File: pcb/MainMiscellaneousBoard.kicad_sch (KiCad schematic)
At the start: 7 parts, among them J4 S04B-PASK-2, J5 Conn_01x08, J6 Conn_01x08, J7 S04B-PASK-2, U1 ItsyBitsy_ESP32, U2 Seeed_Studio_XIAO-ESP32-S3-Se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

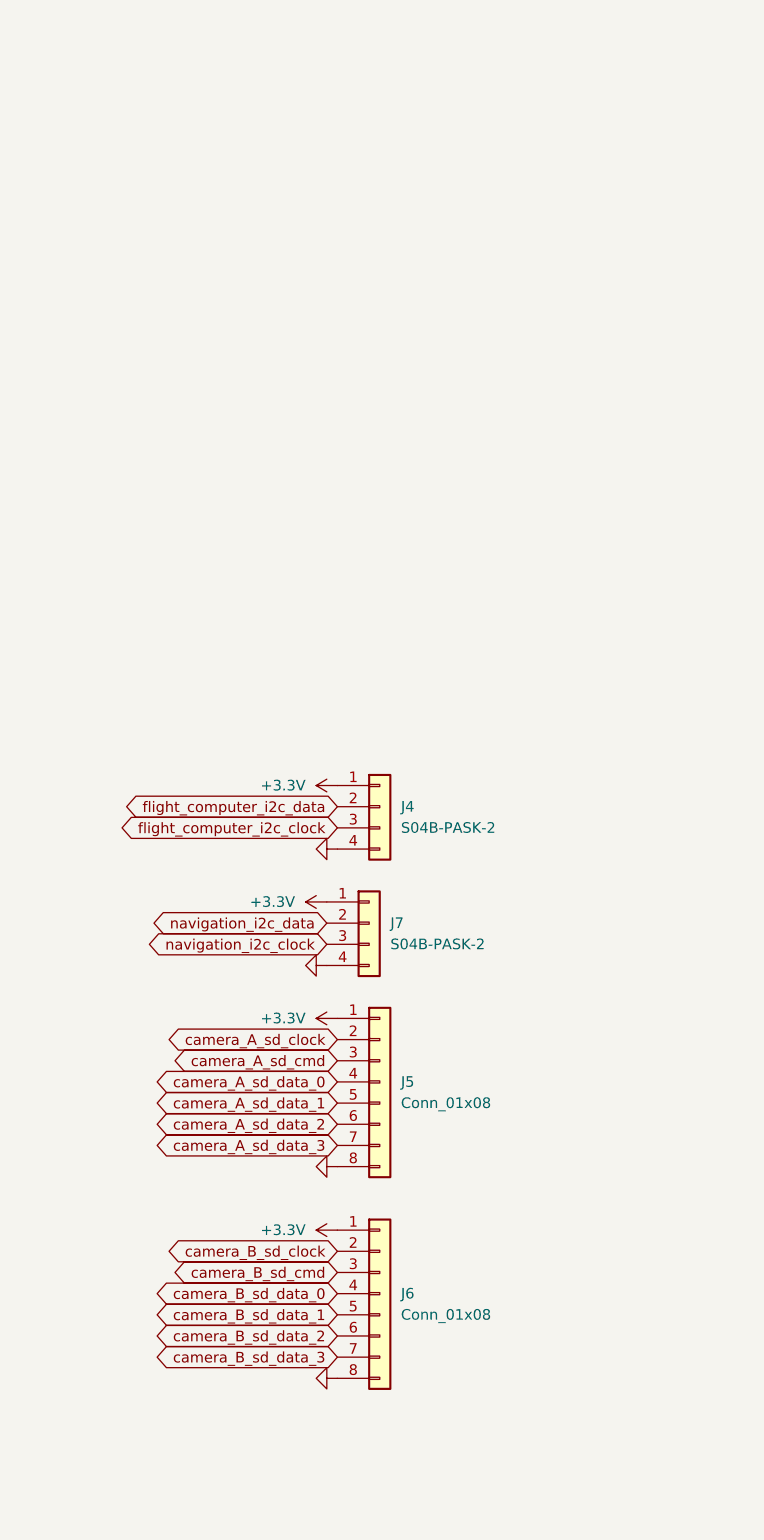
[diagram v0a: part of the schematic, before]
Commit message: Added edge connector for `MainMiscellaneousBoard`.
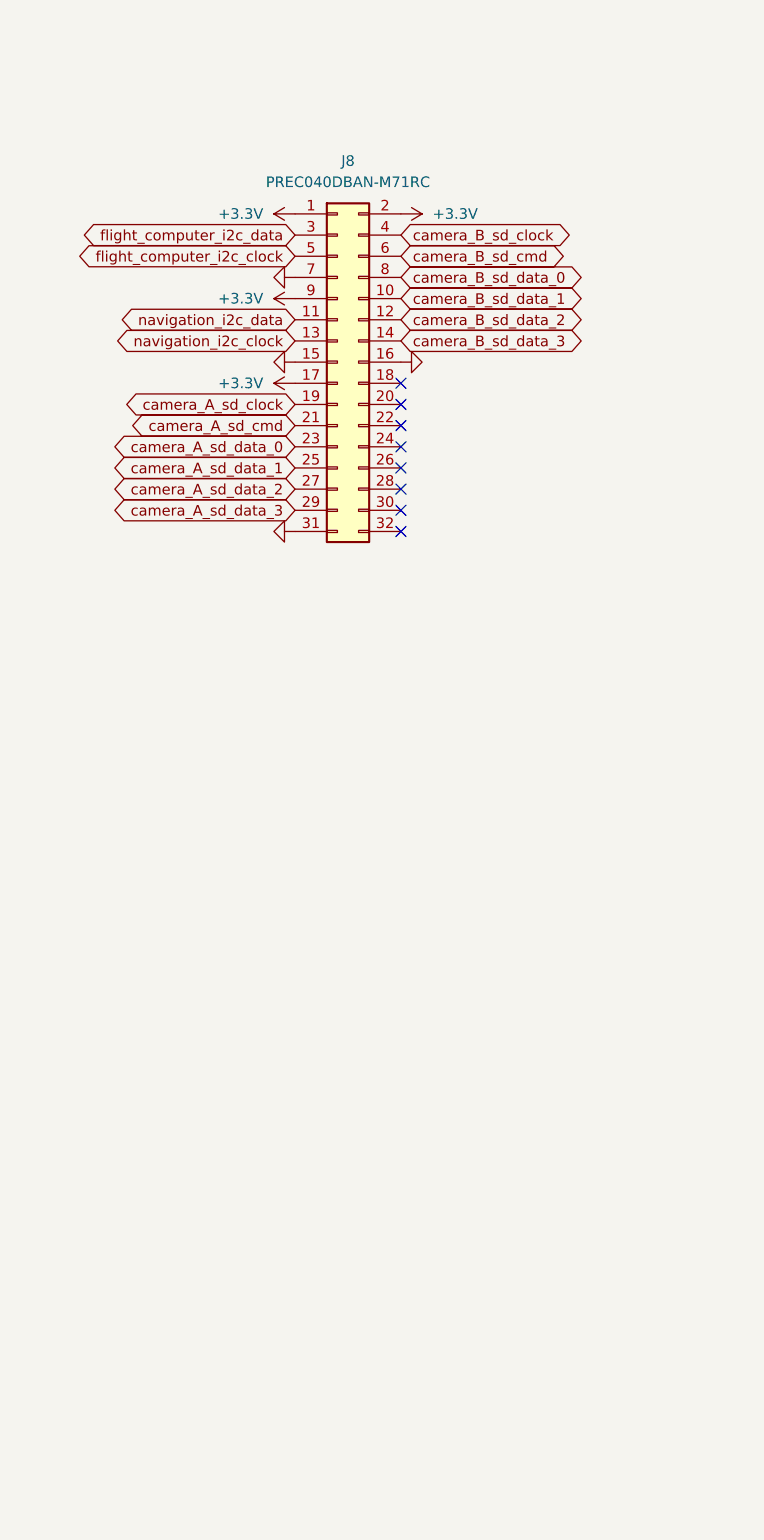
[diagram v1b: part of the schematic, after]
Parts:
- removed J4, J7: S04B-PASK-2, pcb:S04B-PASK-2, symbol Connector_Generic:Conn_01x04
- removed J5, J6: Conn_01x08, symbol Connector_Generic:Conn_01x08
- added J8: PREC040DBAN-M71RC, Connector_PinHeader_2.54mm:PinHeader_2x16_P2.54mm_Horizontal, symbol Connector_Generic:Conn_02x16_Odd_Even
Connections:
- net +3.3V: now also J8.1 (Pin_1), J8.17 (Pin_17), J8.2 (Pin_2), J8.9 (Pin_9)
- net GND: now also J8.15 (Pin_15), J8.16 (Pin_16), J8.31 (Pin_31), J8.7 (Pin_7)
- net camera_A_sd_clock: now also J8.19 (Pin_19)
- net camera_A_sd_cmd: now also J8.21 (Pin_21)
- net camera_A_sd_data_0: now also J8.23 (Pin_23)
- net camera_A_sd_data_1: now also J8.25 (Pin_25)
- net camera_A_sd_data_2: now also J8.27 (Pin_27)
- net camera_A_sd_data_3: now also J8.29 (Pin_29)
- net camera_B_sd_clock: now also J8.4 (Pin_4)
- net camera_B_sd_cmd: now also J8.6 (Pin_6)
- net camera_B_sd_data_0: now also J8.8 (Pin_8)
- net camera_B_sd_data_1: now also J8.10 (Pin_10)
- net camera_B_sd_data_2: now also J8.12 (Pin_12)
- net camera_B_sd_data_3: now also J8.14 (Pin_14)
- net flight_computer_i2c_clock: now also J8.5 (Pin_5)
- net flight_computer_i2c_data: now also J8.3 (Pin_3)
- net navigation_i2c_clock: now also J8.13 (Pin_13)
- net navigation_i2c_data: now also J8.11 (Pin_11)
- no-connect marks 144 -> 152
